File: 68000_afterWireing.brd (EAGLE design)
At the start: 100 x 80 mm, 19 parts, among them IC1 74LS32N, IC2 74LS04N, IC3 74LS04N, X1 22-23-2021

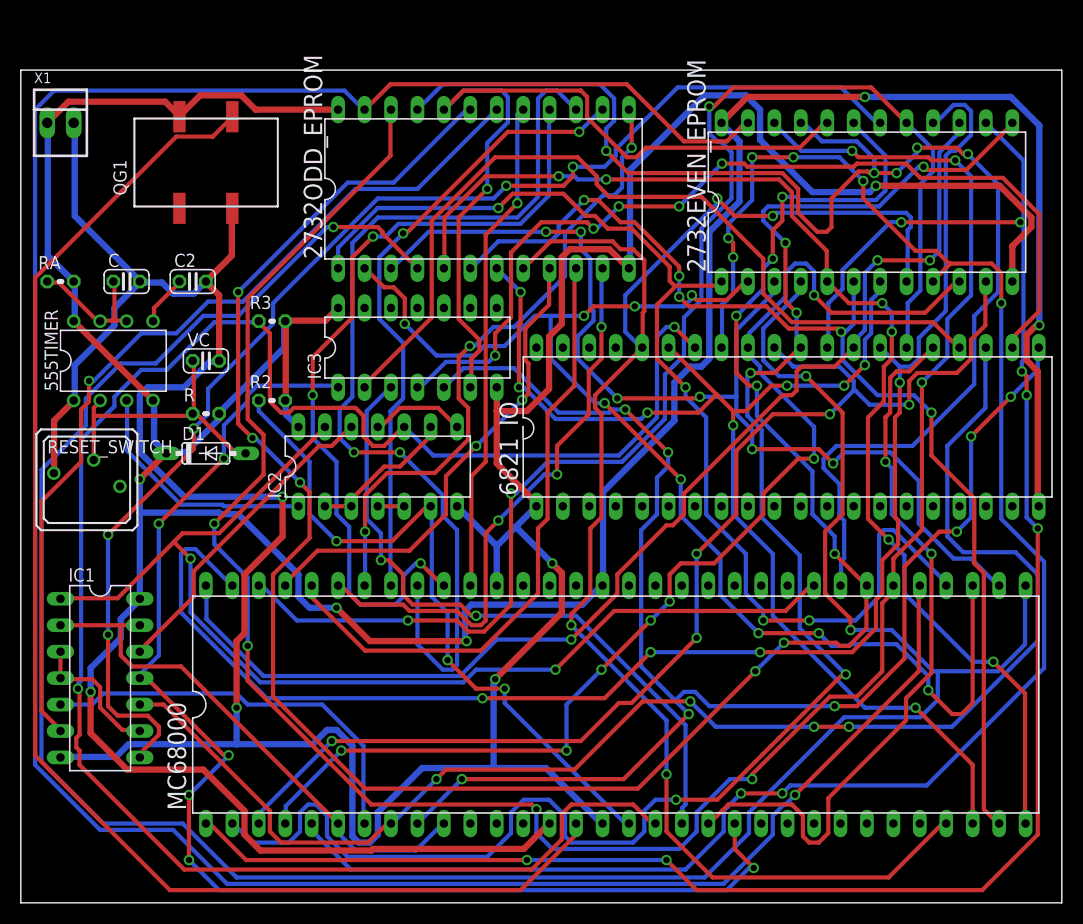
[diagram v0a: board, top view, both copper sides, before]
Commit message: FINAL: Sent to Bay Area Circuits
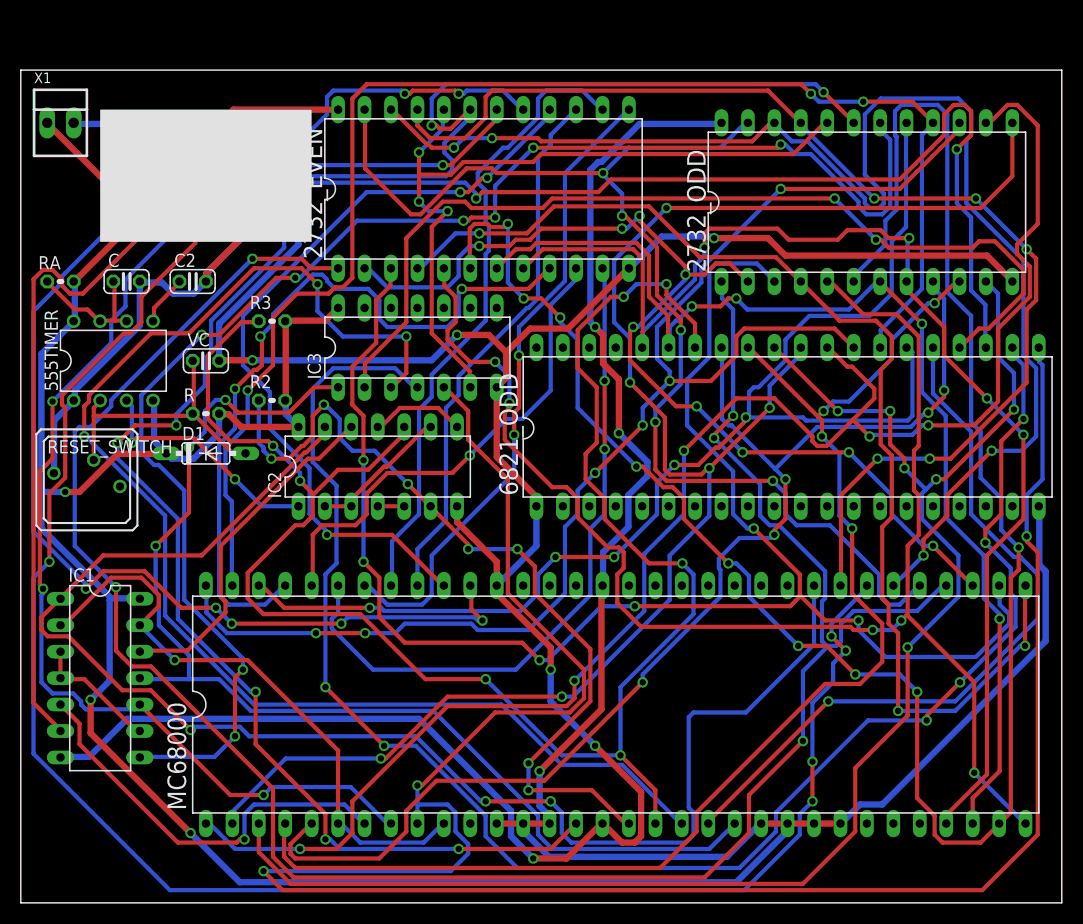
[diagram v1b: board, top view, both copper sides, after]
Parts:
- removed QG1: SG-615PTW, crystal:SG-615
- added U$1: TTL_OSCILLATOR, TTL_OSCILLATOR:TTL_OSCILLATOR
- renumbered 2732EVEN_EPROM to 2732_ODD, 2732ODD_EPROM to 2732_EVEN, 6821_IO to 6821_ODD
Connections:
- net GND: now also U$1.P$7; no longer QG1.2
- net N$26: now also U$1.P$8; no longer QG1.3
- net VCC: now also MC68000.12, MC68000.13, MC68000.22, MC68000.23, MC68000.24, MC68000.25, U$1.P$14; no longer QG1.4
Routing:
- net A5: track 245.3 -> 111.7 mm
- net A9: track 244.5 -> 115.0 mm, vias 1 -> 5
- net A8: track 109.7 -> 208.4 mm, vias 4 -> 5
- net A3: track 106.9 -> 192.9 mm, vias 5 -> 9
- net D15: track 47.9 -> 132.5 mm, vias 1 -> 7
- net A10: track 214.1 -> 130.6 mm, vias 7 -> 4
- net N$1: track 145.5 -> 212.8 mm, vias 8 -> 3
- net N$11: track 90.2 -> 157.2 mm, vias 5 -> 6
- net N$12: track 64.8 -> 127.9 mm, vias 2 -> 3
- net N$9: track 139.3 -> 198.3 mm, vias 4 -> 5
- net D0: track 173.3 -> 119.1 mm, vias 8 -> 5
- net A6: track 100.6 -> 153.6 mm
- net A11: track 207.3 -> 252.4 mm, vias 10 -> 8
- net D13: track 92.8 -> 52.1 mm, vias 2 -> 0
- net N$3: track 106.3 -> 141.4 mm, vias 2 -> 3
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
